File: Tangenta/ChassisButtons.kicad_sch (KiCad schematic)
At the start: 19 parts, among them J2 Conn_02x02_Top_Bottom, Q1 2N7002, Q2 2N7002, U5 74HC74D,653, U6 CD4060SA_TR, U7 74HC04D,653

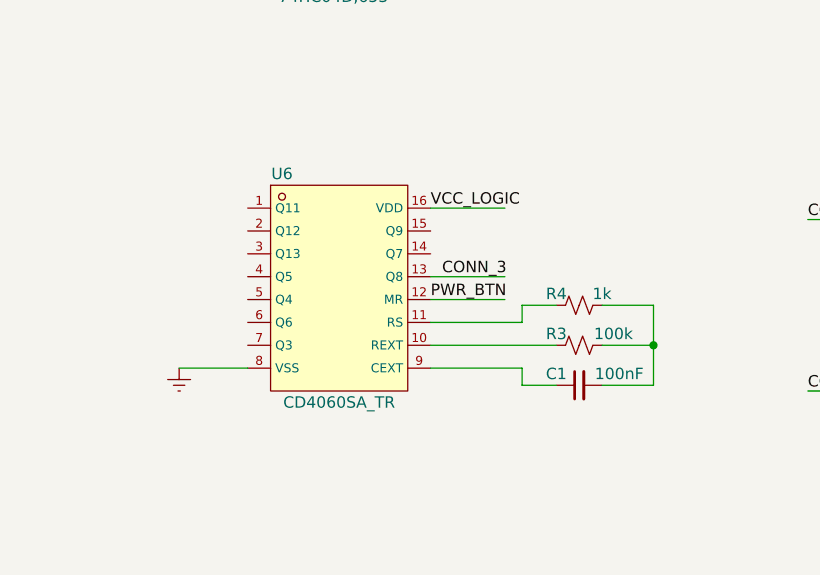
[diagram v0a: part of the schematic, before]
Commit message: Power supply - current progress.
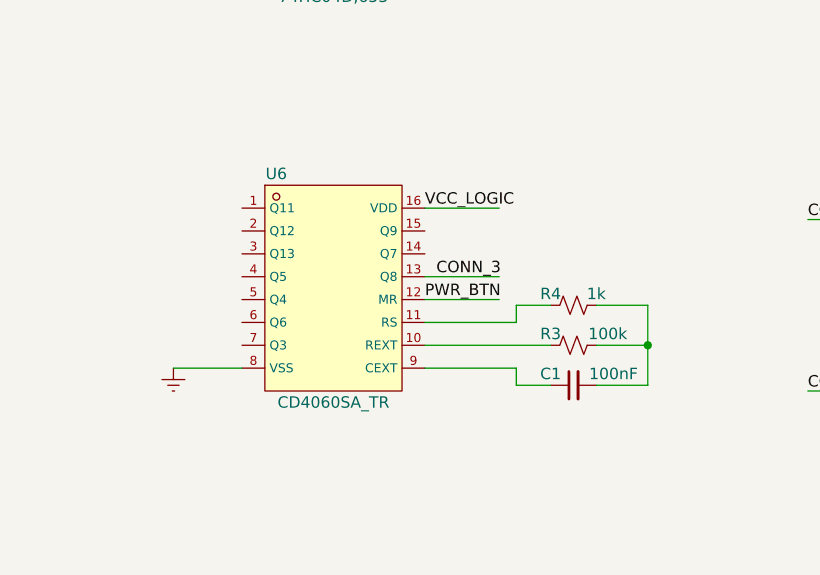
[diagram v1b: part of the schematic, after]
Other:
- moved on the sheet: C1, R3, R4, U6
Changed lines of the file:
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@@
   (junction (at 68.58 68.58) (diameter 0) (color 0 0 0 0)
   )
-  (junction (at 177.165 116.205) (diameter 0) (color 0 0 0 0)
+  (junction (at 176.53 116.205) (diameter 0) (color 0 0 0 0)
   )
   (junction (at 211.455 121.285) (diameter 0) (color 0 0 0 0)
@@
     (stroke (width 0) (type default))
   )
-  (wire (pts (xy 152.4 116.205) (xy 166.37 116.205))
+  (wire (pts (xy 151.765 116.205) (xy 165.735 116.205))
     (stroke (width 0) (type default))
   )
@@
     (stroke (width 0) (type default))
   )
-  (wire (pts (xy 152.4 100.965) (xy 160.655 100.965))
+  (wire (pts (xy 151.765 100.965) (xy 160.02 100.965))
     (stroke (width 0) (type default))
   )
@@
     (stroke (width 0) (type default))
   )
-  (wire (pts (xy 152.4 111.125) (xy 160.655 111.125))
+  (wire (pts (xy 151.765 111.125) (xy 160.02 111.125))
     (stroke (width 0) (type default))
   )
@@
     (stroke (width 0) (type default))
   )
-  (wire (pts (xy 152.4 108.585) (xy 160.655 108.585))
-    (stroke (width 0) (type default))
-  )
-  (wire (pts (xy 177.165 111.76) (xy 177.165 116.205))
+  (wire (pts (xy 151.765 108.585) (xy 160.02 108.585))
+    (stroke (width 0) (type default))
+  )
+  (wire (pts (xy 176.53 111.76) (xy 176.53 116.205))
     (stroke (width 0) (type default))
   )
@@
     (stroke (width 0) (type default))
   )
-  (wire (pts (xy 162.56 120.65) (xy 166.37 120.65))
+  (wire (pts (xy 161.925 120.65) (xy 165.735 120.65))
     (stroke (width 0) (type default))
   )
@@
     (stroke (width 0) (type default))
   )
-  (wire (pts (xy 177.165 120.65) (xy 171.45 120.65))
-    (stroke (width 0) (type default))
-  )
-  (wire (pts (xy 124.46 118.745) (xy 132.08 118.745))
+  (wire (pts (xy 176.53 120.65) (xy 170.815 120.65))
+    (stroke (width 0) (type default))
+  )
+  (wire (pts (xy 123.825 118.745) (xy 131.445 118.745))
     (stroke (width 0) (type default))
   )
@@
     (stroke (width 0) (type default))
   )
-  (wire (pts (xy 152.4 113.665) (xy 162.56 113.665))
+  (wire (pts (xy 151.765 113.665) (xy 161.925 113.665))
     (stroke (width 0) (type default))
   )
@@
     (stroke (width 0) (type default))
   )
-  (wire (pts (xy 162.56 118.745) (xy 162.56 120.65))
-    (stroke (width 0) (type default))
-  )
-  (wire (pts (xy 171.45 116.205) (xy 177.165 116.205))
+  (wire (pts (xy 161.925 118.745) (xy 161.925 120.65))
+    (stroke (width 0) (type default))
+  )
+  (wire (pts (xy 170.815 116.205) (xy 176.53 116.205))
     (stroke (width 0) (type default))
   )
@@
     (stroke (width 0) (type default))
   )
-  (wire (pts (xy 171.45 111.76) (xy 177.165 111.76))
+  (wire (pts (xy 170.815 111.76) (xy 176.53 111.76))
     (stroke (width 0) (type default))
   )
@@
     (stroke (width 0) (type default))
   )
-  (wire (pts (xy 152.4 118.745) (xy 162.56 118.745))
-    (stroke (width 0) (type default))
-  )
-  (wire (pts (xy 177.165 116.205) (xy 177.165 120.65))
-    (stroke (width 0) (type default))
-  )
-  (wire (pts (xy 162.56 113.665) (xy 162.56 111.76))
+  (wire (pts (xy 151.765 118.745) (xy 161.925 118.745))
+    (stroke (width 0) (type default))
+  )
+  (wire (pts (xy 176.53 116.205) (xy 176.53 120.65))
+    (stroke (width 0) (type default))
+  )
+  (wire (pts (xy 161.925 113.665) (xy 161.925 111.76))
     (stroke (width 0) (type default))
   )
@@
     (stroke (width 0) (type default))
   )
-  (wire (pts (xy 162.56 111.76) (xy 166.37 111.76))
+  (wire (pts (xy 161.925 111.76) (xy 165.735 111.76))
     (stroke (width 0) (type default))
   )
@@
     (effects (font (size 1.27 1.27)) (justify right bottom))
   )
-  (label "PWR_BTN" (at 152.4 111.125 0) (fields_autoplaced)
+  (label "PWR_BTN" (at 151.765 111.125 0) (fields_autoplaced)
     (effects (font (size 1.27 1.27)) (justify left bottom))
   )
@@
     (effects (font (size 1.27 1.27)) (justify left bottom))
   )
-  (label "VCC_LOGIC" (at 152.4 100.965 0) (fields_autoplaced)
+  (label "VCC_LOGIC" (at 151.765 100.965 0) (fields_autoplaced)
     (effects (font (size 1.27 1.27)) (justify left bottom))
   )
@@
     (effects (font (size 1.27 1.27)) (justify left bottom))
   )
-  (label "CONN_3" (at 153.67 108.585 0) (fields_autoplaced)
+  (label "CONN_3" (at 153.035 108.585 0) (fields_autoplaced)
     (effects (font (size 1.27 1.27)) (justify left bottom))
   )
@@
     )
   )
-  (symbol (lib_id "Device:R_Small_US") (at 168.91 116.205 90) (unit 1)
-    (in_bom yes) (on_board yes) (dnp no)
-    (property "Reference" "R3" (at 166.37 114.935 90)
-      (effects (font (size 1.27 1.27)))
-    )
-    (property "Value" "100k" (at 172.72 114.935 90)
-      (effects (font (size 1.27 1.27)))
-    )
-    (property "Footprint" "Resistor_SMD:R_0603_1608Metric" (at 168.91 116.205 0)
-      (effects (font (size 1.27 1.27)) hide)
-    )
-    (property "Datasheet" "~" (at 168.91 116.205 0)
+  (symbol (lib_id "Device:R_Small_US") (at 168.275 116.205 90) (unit 1)
+    (in_bom yes) (on_board yes) (dnp no)
+    (property "Reference" "R3" (at 165.735 114.935 90)
+      (effects (font (size 1.27 1.27)))
+    )
+    (property "Value" "100k" (at 172.085 114.935 90)
+      (effects (font (size 1.27 1.27)))
+    )
+    (property "Footprint" "Resistor_SMD:R_0603_1608Metric" (at 168.275 116.205 0)
+      (effects (font (size 1.27 1.27)) hide)
+    )
+    (property "Datasheet" "~" (at 168.275 116.205 0)
       (effects (font (size 1.27 1.27)) hide)
     )
@@
     )
   )
-  (symbol (lib_id "CD4060:CD4060SA_TR") (at 142.24 109.855 0) (unit 1)
-    (in_bom yes) (on_board yes) (dnp no)
-    (property "Reference" "U6" (at 135.89 97.155 0)
-      (effects (font (size 1.27 1.27)))
-    )
-    (property "Value" "CD4060SA_TR" (at 142.24 122.555 0)
-      (effects (font (size 1.27 1.27)))
-    )
-    (property "Footprint" "CD4060:CD4060" (at 142.24 128.524 0)
+  (symbol (lib_id "CD4060:CD4060SA_TR") (at 141.605 109.855 0) (unit 1)
+    (in_bom yes) (on_board yes) (dnp no)
+    (property "Reference" "U6" (at 135.255 97.155 0)
+      (effects (font (size 1.27 1.27)))
+    )
+    (property "Value" "CD4060SA_TR" (at 141.605 122.555 0)
+      (effects (font (size 1.27 1.27)))
+    )
+    (property "Footprint" "CD4060:CD4060" (at 141.605 128.524 0)
       (effects (font (size 1.27 1.27) italic) hide)
     )
-    (property "Datasheet" "http://datasheet.octopart.com/MC14076BDR2G-ON-Semiconductor-datasheet-608107.pdf" (at 134.874 130.81 0)
+    (property "Datasheet" "http://datasheet.octopart.com/MC14076BDR2G-ON-Semiconductor-datasheet-608107.pdf" (at 134.239 130.81 0)
       (effects (font (size 1.27 1.27)) (justify left) hide)
     )
-    (property "LCSC" "C2943323" (at 139.446 126.238 0)
+    (property "LCSC" "C2943323" (at 138.811 126.238 0)
       (effects (font (size 1.27 1.27)) hide)
     )
@@
     )
   )
-  (symbol (lib_id "Device:R_Small_US") (at 168.91 111.76 90) (unit 1)
-    (in_bom yes) (on_board yes) (dnp no)
-    (property "Reference" "R4" (at 166.37 110.49 90)
-      (effects (font (size 1.27 1.27)))
-    )
-    (property "Value" "1k" (at 171.45 110.49 90)
-      (effects (font (size 1.27 1.27)))
-    )
-    (property "Footprint" "Resistor_SMD:R_0603_1608Metric" (at 168.91 111.76 0)
-      (effects (font (size 1.27 1.27)) hide)
-    )
-    (property "Datasheet" "~" (at 168.91 111.76 0)
+  (symbol (lib_id "Device:R_Small_US") (at 168.275 111.76 90) (unit 1)
+    (in_bom yes) (on_board yes) (dnp no)
+    (property "Reference" "R4" (at 165.735 110.49 90)
+      (effects (font (size 1.27 1.27)))
+    )
+    (property "Value" "1k" (at 170.815 110.49 90)
+      (effects (font (size 1.27 1.27)))
+    )
+    (property "Footprint" "Resistor_SMD:R_0603_1608Metric" (at 168.275 111.76 0)
+      (effects (font (size 1.27 1.27)) hide)
+    )
+    (property "Datasheet" "~" (at 168.275 111.76 0)
       (effects (font (size 1.27 1.27)) hide)
     )
@@
     )
   )
-  (symbol (lib_id "Device:C_Small") (at 168.91 120.65 90) (unit 1)
-    (in_bom yes) (on_board yes) (dnp no)
-    (property "Reference" "C1" (at 166.37 119.38 90)
-      (effects (font (size 1.27 1.27)))
-    )
-    (property "Value" "100nF" (at 173.355 119.38 90)
-      (effects (font (size 1.27 1.27)))
-    )
-    (property "Footprint" "" (at 168.91 120.65 0)
-      (effects (font (size 1.27 1.27)) hide)
-    )
-    (property "Datasheet" "~" (at 168.91 120.65 0)
+  (symbol (lib_id "Device:C_Small") (at 168.275 120.65 90) (unit 1)
+    (in_bom yes) (on_board yes) (dnp no)
+    (property "Reference" "C1" (at 165.735 119.38 90)
+      (effects (font (size 1.27 1.27)))
+    )
+    (property "Value" "100nF" (at 172.72 119.38 90)
+      (effects (font (size 1.27 1.27)))
+    )
+    (property "Footprint" "" (at 168.275 120.65 0)
+      (effects (font (size 1.27 1.27)) hide)
+    )
+    (property "Datasheet" "~" (at 168.275 120.65 0)
       (effects (font (size 1.27 1.27)) hide)
     )
@@
     )
   )
-  (symbol (lib_id "power:GNDREF") (at 124.46 118.745 0) (unit 1)
-    (in_bom yes) (on_board yes) (dnp no) (fields_autoplaced)
-    (property "Reference" "#PWR06" (at 124.46 125.095 0)
-      (effects (font (size 1.27 1.27)) hide)
-    )
-    (property "Value" "GNDREF" (at 124.46 123.825 0)
-      (effects (font (size 1.27 1.27)) hide)
-    )
-    (property "Footprint" "" (at 124.46 118.745 0)
-      (effects (font (size 1.27 1.27)) hide)
-    )
-    (property "Datasheet" "" (at 124.46 118.745 0)
-      (effects (font (size 1.27 1.27)) hide)
-    )
+  (symbol (lib_id "power:GNDREF") (at 123.825 118.745 0) (unit 1)
+    (in_bom yes) (on_board yes) (dnp no) (fields_autoplaced)
+    (property "Reference" "#PWR06" (at 123.825 125.095 0)
+      (effects (font (size 1.27 1.27)) hide)
+    )
+    (property "Value" "GNDREF" (at 123.825 123.825 0)
+      (effects (font (size 1.27 1.27)) hide)
+    )
+    (property "Footprint" "" (at 123.825 118.745 0)
+      (effects (font (size 1.27 1.27)) hide)
+    )
+    (property "Datasheet" "" (at 123.825 118.745 0)
+      (effects (font (size 1.27 1.27)) hide)
+    )

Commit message: Current progress...
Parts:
- C1, C3, C4: footprint (none) -> Capacitor_SMD:C_0603_1608Metric
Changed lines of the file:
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@@
       (effects (font (size 1.27 1.27)))
     )
-    (property "Footprint" "" (at 69.215 111.125 0)
+    (property "Footprint" "Capacitor_SMD:C_0603_1608Metric" (at 69.215 111.125 0)
       (effects (font (size 1.27 1.27)) hide)
     )
@@
       (effects (font (size 1.27 1.27)))
     )
-    (property "Footprint" "" (at 168.275 120.65 0)
+    (property "Footprint" "Capacitor_SMD:C_0603_1608Metric" (at 168.275 120.65 0)
       (effects (font (size 1.27 1.27)) hide)
     )
@@
       (effects (font (size 1.27 1.27)))
     )
-    (property "Footprint" "" (at 78.74 111.125 0)
-      (effects (font (size 1.27 1.27)) hide)
-    )
+    (property "Footprint" "Capacitor_SMD:C_0603_1608Metric" (at 78.74 111.125 0)
+      (effects (font (size 1.27 1.27)) hide)
+    )
